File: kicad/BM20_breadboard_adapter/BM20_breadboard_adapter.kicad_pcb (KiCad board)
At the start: 2 copper layers, 29.5 x 47.2 mm, 24 parts, among them CON1 CONN_18, CON2 CONN_18, CON3 batt, J1 PJ-320B, J2 PJ-320B, J3 USB_B_Micro, SW1 SWITCH_SPST, SW2 SWITCH_SPST, U1 BM20

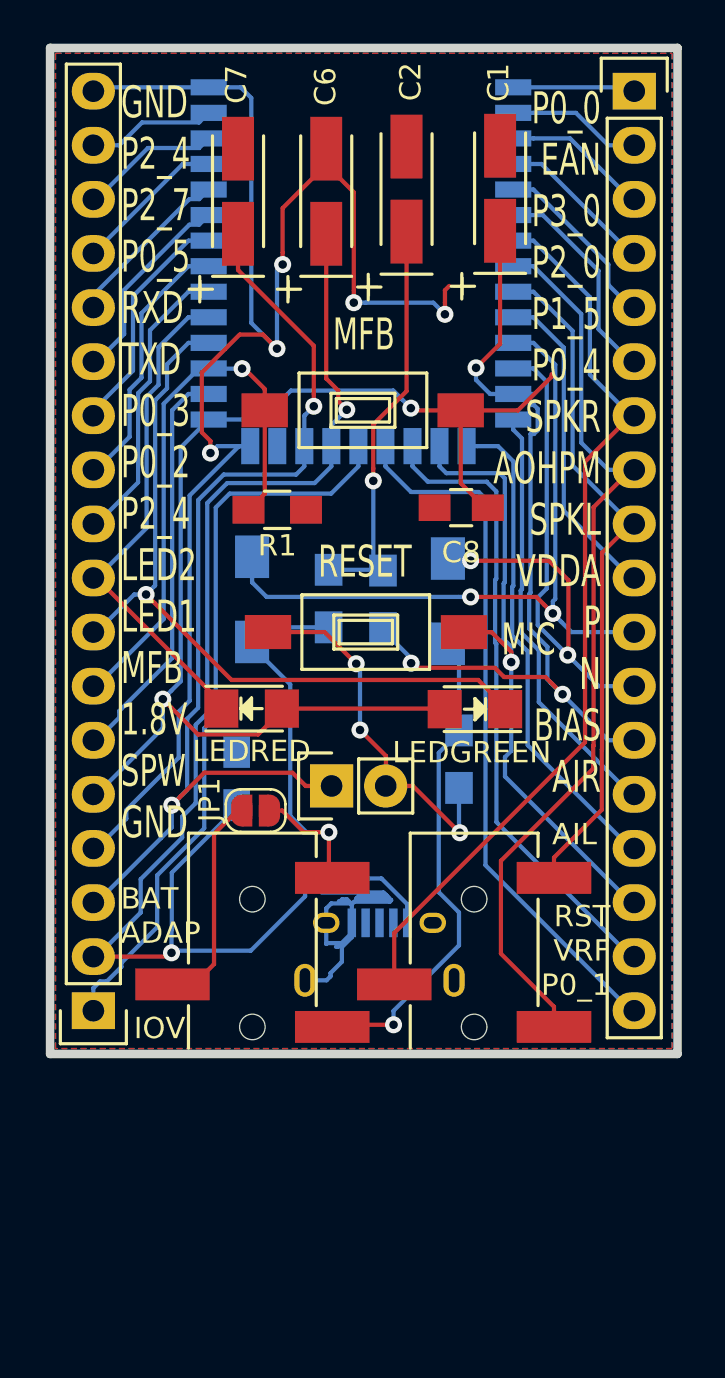
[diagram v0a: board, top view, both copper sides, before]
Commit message: update
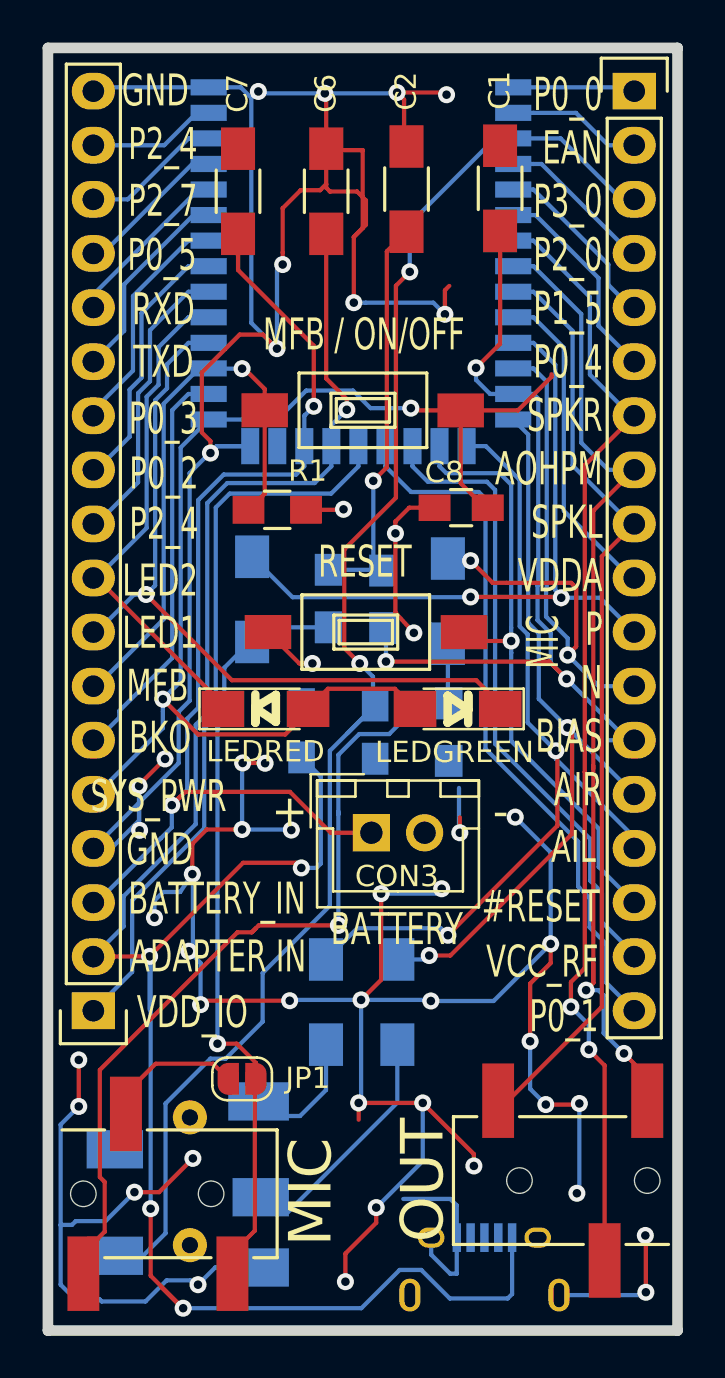
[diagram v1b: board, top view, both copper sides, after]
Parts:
- added C10: 10uF/16V, Capacitors_SMD.pretty:C_1206_HandSoldering, B.Cu at (141.3, 93.6)
- added C11: 10u/16V, Capacitors_SMD.pretty:C_1206_HandSoldering, B.Cu at (137.9, 93.6)
- added C9: 100n, Capacitors_SMD.pretty:C_0805_HandSoldering, B.Cu at (140.2, 80.9)
- added U2: PJ-3027F, jacks:PJ-3027F-S, B.Cu at (131.5, 108.0)
- C1, C2: value 2.2u/6.3V -> 1u/16V; footprint Capacitors_Tantalum_SMD.pretty:TantalC_SizeA_EIA-3216_HandSoldering -> Capacitors_SMD.pretty:C_1206_HandSoldering
- C3, C4: value 1u/16V -> 0,1u/16V
- C6, C7: value 10u/16V/PacA/AVX -> 10u/16V; footprint Capacitors_Tantalum_SMD.pretty:TantalC_SizeA_EIA-3216_HandSoldering -> Capacitors_SMD.pretty:C_1206_HandSoldering
- CON3: footprint Pin_Headers.pretty:Pin_Header_Straight_1x02 -> Connectors_JST:JST_XH_B02B-XH-A_02x2.50mm_Straight
- D1, D2: footprint LEDs.pretty:LED-1206 -> LEDs:LED_1206_HandSoldering
- moved J3 15.6 mm to (145.4, 106.2)
- moved JP1 12.6 mm to (134.0, 97.2)
- moved J2 11.2 mm to (126.5, 102.6), turned to 90 degrees
- moved J1 10.9 mm to (153.0, 102.0), turned to -90 degrees
- moved C5 3.78 mm to (136.8, 80.8)
- moved CON3 2.88 mm to (140.1, 85.6), turned to 0 degrees
- moved R4 1.36 mm to (143.7, 80.9)
- moved D1 0.81 mm to (144.1, 79.8)
- moved D2 0.65 mm to (135.1, 79.8)
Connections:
- U1 pad 22: /GND -> (no net)
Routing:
- net /GND: track 113.2 -> 254.0 mm, vias 8 -> 48
- net /3: track 6.87 -> 70.5 mm, vias 0 -> 2
- net /20: track 68.1 -> 101.3 mm, vias 2 -> 5
- net Net-(C4-Pad2): track 23.1 -> 42.3 mm
- net /15: track 23.2 -> 40.1 mm, vias 0 -> 2
- net Net-(C3-Pad2): track 20.3 -> 36.0 mm
- net /14: track 20.1 -> 35.7 mm, vias 0 -> 2
- net /9: track 32.2 -> 43.9 mm
- net Net-(C10-Pad2): track 0.00 -> 11.4 mm
- net /7: track 42.7 -> 52.8 mm, vias 0 -> 2
- net Net-(C11-Pad1): track 0.00 -> 6.06 mm
- net Net-(J2-Pad3): track 10.5 -> 5.91 mm
- net /8: track 43.1 -> 46.3 mm, vias 0 -> 2
- net /21: track 47.6 -> 50.2 mm
- net /16: track 30.1 -> 29.1 mm
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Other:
- board size 29.5 x 47.2 mm -> 29.6 x 60.2 mm
- board text added: "#RESET"
- board text added: "+"
- board text added: "-"
- board text added: "ADAPTER IN"
- board text added: "AUX"
- board text added: "BATTERY"
- board text added: "BATTERY_IN"
- board text added: "BKO"
- board text added: "GND"
- board text added: "LED1"
- board text added: "LED2"
- board text added: "MFB / ON/OFF"
- board text added: "OUT"
- board text added: "P0_1"
- board text added: "P0_2"
- board text added: "P0_3"
- board text added: "P0_5"
- board text added: "P2_4"
- board text added: "P2_7"
- board text added: "POWER"
- board text added: "RXD"
- board text added: "SYS_PWR"
- board text added: "TXD"
- board text added: "VCC_RF"
- board text added: "VDD_IO"
- board text removed: "BAT ADAP"
- board text removed: "GND P2_4 P2_7 P0_5 RXD TXD P0_3 P0_2 P2_4 LED2 LED1 MFB 1.8V SPW GND"
- board text removed: "IOV"
- board text removed: "RST VRF P0_1"
